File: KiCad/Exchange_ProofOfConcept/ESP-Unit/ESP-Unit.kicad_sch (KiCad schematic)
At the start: 52 parts, among them IC1 MT8870DE, J1 Jack-DC, J2 Conn_02x05_Top_Bottom, J3 Conn_01x07, U1 ESP32_NODEMCU, U2 LM317_TO-220, U3 LM358PE3, U4 BOB-12009, U5 BOB-12009, Y1 3.579546

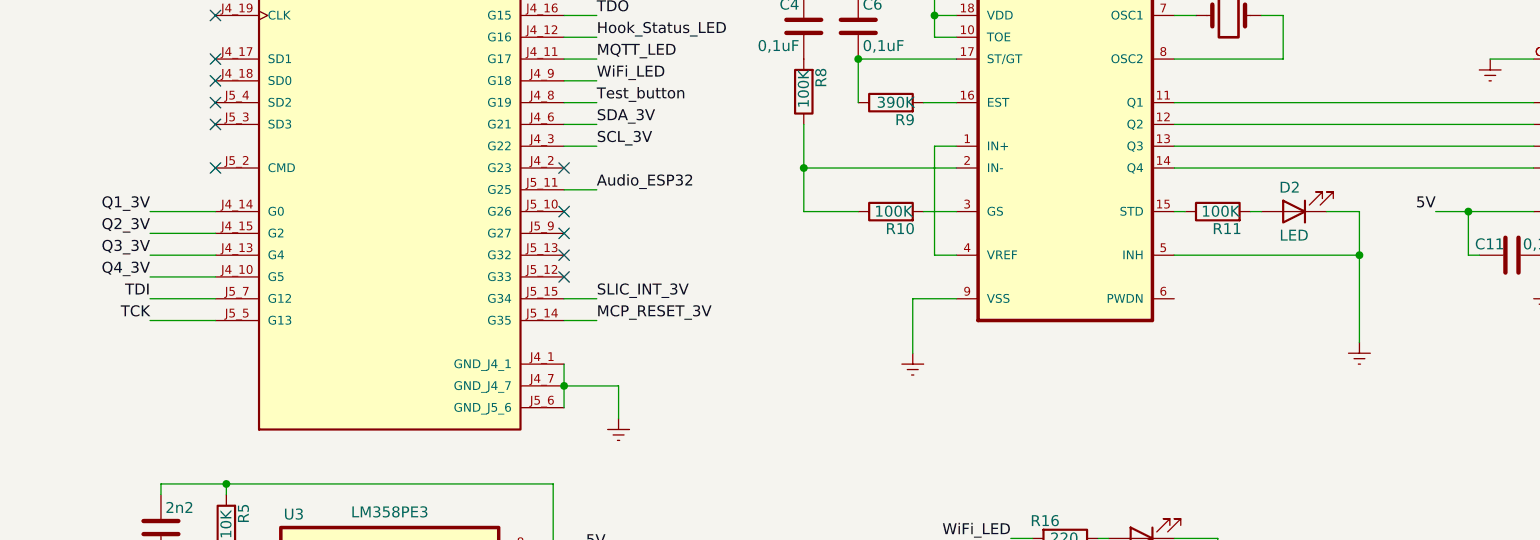
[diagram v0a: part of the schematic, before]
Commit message: modified:   KiCad/Exchange_ProofOfConcept/ESP-Unit/ESP-Unit.kicad_sch 	deleted:    KiCad/Exchange_ProofOfConcept/ESP-Unit/_autosave-ESP-Unit.kicad_sch 	modified:   include/config.h 	new file:   include/toneHandler.h 	modified:   lib/MT8816/MT8816.cpp 	modified:   src/config.cpp 	modified:   src/hookChange.cpp 	modified:   src/lineAction.cpp 	modified:   src/main.cpp 	new file:   src/toneHandler.cpp
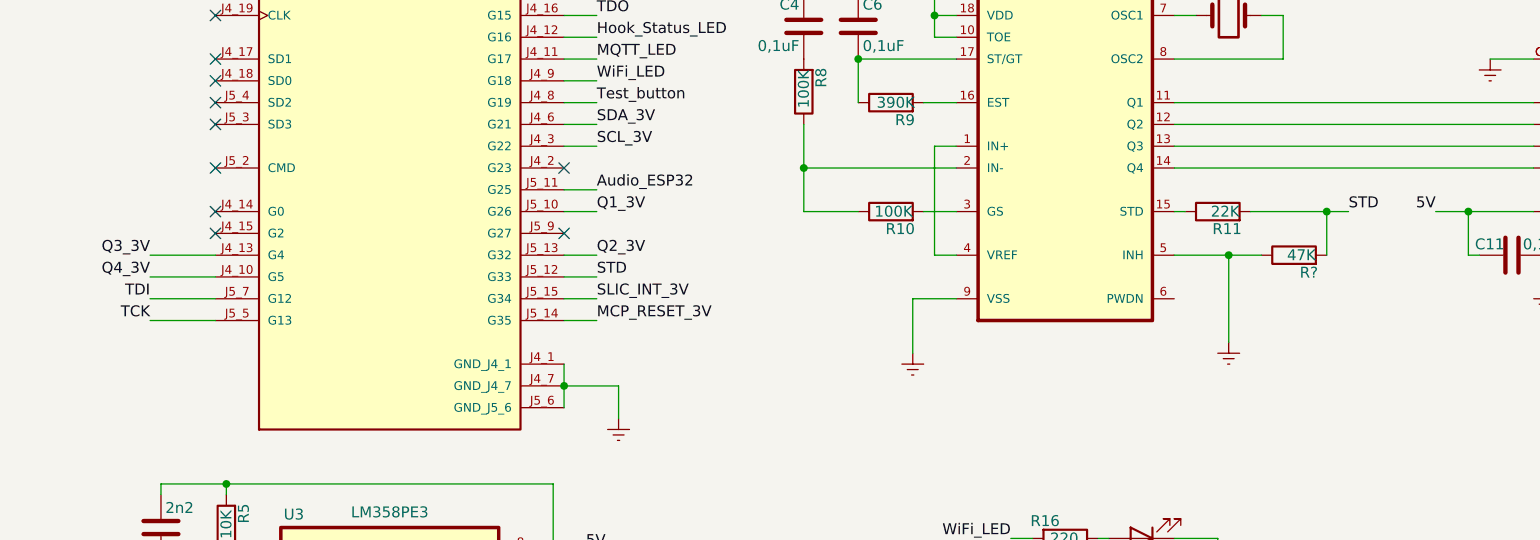
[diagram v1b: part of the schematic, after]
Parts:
- removed D2: LED, LED_THT:LED_D3.0mm, symbol Device:LED
- added R?: 47K, Resistor_THT:R_Axial_DIN0207_L6.3mm_D2.5mm_P2.54mm_Vertical, symbol Device:R
- R11: value 100K -> 22K
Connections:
- net Earth: now also R?.1
- net Q1_3V: now also U1.J5_10 (G26); no longer U1.J4_14 (G0)
- net Q2_3V: now also U1.J5_13 (G32); no longer U1.J4_15 (G2)
- net STD: now reaches R11.2
- net STD: now also U1.J5_12 (G33), R?.2
- no-connect marks 17 -> 16
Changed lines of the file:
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@@
 	)
 	(junction
+		(at 156.21 128.27)
+		(diameter 0)
+		(color 0 0 0 0)
+	)
+	(junction
 		(at 39.37 170.18)
 		(diameter 0)
@@
 	)
 	(junction
-		(at 171.45 128.27)
+		(at 167.64 123.19)
 		(diameter 0)
 		(color 0 0 0 0)
@@
 	)
 	(no_connect
+		(at 38.1 125.73)
+	)
+	(no_connect
 		(at 38.1 107.95)
 	)
@@
 	)
 	(no_connect
-		(at 78.74 128.27)
-	)
-	(no_connect
 		(at 38.1 92.71)
 	)
@@
 	)
 	(no_connect
-		(at 78.74 130.81)
-	)
-	(no_connect
 		(at 269.24 151.13)
 	)
@@
 	)
 	(no_connect
+		(at 38.1 123.19)
+	)
+	(no_connect
 		(at 38.1 118.11)
 	)
@@
 		(at 78.74 92.71)
 	)
-	(no_connect
-		(at 78.74 123.19)
-	)
 	(wire
 		(pts
@@
 	(wire
 		(pts
-			(xy 160.02 123.19) (xy 158.75 123.19)
+			(xy 158.75 123.19) (xy 167.64 123.19)
 		)
 		(stroke
@@
 	(wire
 		(pts
+			(xy 167.64 128.27) (xy 167.64 123.19)
+		)
+		(stroke
+			(width 0)
+			(type default)
+		)
+	)
+	(wire
+		(pts
 			(xy 107.95 46.99) (xy 107.95 58.42)
 		)
@@
 	(wire
 		(pts
-			(xy 149.86 128.27) (xy 171.45 128.27)
+			(xy 149.86 128.27) (xy 156.21 128.27)
 		)
 		(stroke
@@
 	(wire
 		(pts
-			(xy 30.48 123.19) (xy 38.1 123.19)
-		)
-		(stroke
-			(width 0)
-			(type default)
-		)
-	)
-	(wire
-		(pts
 			(xy 39.37 175.26) (xy 39.37 177.8)
 		)
@@
 	(wire
 		(pts
-			(xy 30.48 130.81) (xy 38.1 130.81)
+			(xy 167.64 123.19) (xy 170.18 123.19)
 		)
 		(stroke
@@
 	(wire
 		(pts
-			(xy 167.64 123.19) (xy 171.45 123.19)
+			(xy 30.48 130.81) (xy 38.1 130.81)
 		)
 		(stroke
@@
 	(wire
 		(pts
+			(xy 78.74 128.27) (xy 82.55 128.27)
+		)
+		(stroke
+			(width 0)
+			(type default)
+		)
+	)
+	(wire
+		(pts
 			(xy 248.92 73.66) (xy 248.92 83.82)
 		)
@@
 	(wire
 		(pts
+			(xy 78.74 123.19) (xy 82.55 123.19)
+		)
+		(stroke
+			(width 0)
+			(type default)
+		)
+	)
+	(wire
+		(pts
 			(xy 130.81 176.53) (xy 133.35 176.53)
 		)
@@
 	(wire
 		(pts
-			(xy 171.45 128.27) (xy 171.45 138.43)
+			(xy 156.21 128.27) (xy 156.21 138.43)
 		)
 		(stroke
@@
 	(wire
 		(pts
-			(xy 171.45 123.19) (xy 171.45 128.27)
+			(xy 31.75 165.1) (xy 39.37 165.1)
 		)
 		(stroke
@@
 	(wire
 		(pts
-			(xy 31.75 165.1) (xy 39.37 165.1)
+			(xy 78.74 130.81) (xy 82.55 130.81)
 		)
 		(stroke
@@
 	(wire
 		(pts
+			(xy 156.21 128.27) (xy 160.02 128.27)
+		)
+		(stroke
+			(width 0)
+			(type default)
+		)
+	)
+	(wire
+		(pts
 			(xy 120.65 110.49) (xy 124.46 110.49)
 		)
@@
 	(wire
 		(pts
-			(xy 30.48 125.73) (xy 38.1 125.73)
-		)
-		(stroke
-			(width 0)
-			(type default)
-		)
-	)
-	(wire
-		(pts
 			(xy 74.93 50.8) (xy 83.82 50.8)
 		)
@@
 		)
 	)
+	(label "STD"
+		(at 82.55 130.81 0)
+		(effects
+			(font
+				(size 1.27 1.27)
+			)
+			(justify left bottom)
+		)
+	)
 	(label "3V3"
 		(at 92.71 85.09 0)
@@
 		)
 	)
+	(label "STD"
+		(at 170.18 123.19 0)
+		(effects
+			(font
+				(size 1.27 1.27)
+			)
+			(justify left bottom)
+		)
+	)
 	(label "5V"
 		(at 118.11 86.36 180)
@@
 		)
 	)
-	(label "Q2_3V"
-		(at 30.48 125.73 180)
-		(effects
-			(font
-				(size 1.27 1.27)
-			)
-			(justify right bottom)
-		)
-	)
 	(label "Audio_SLIC-Amp"
 		(at 81.28 167.64 0)
@@
 		)
 	)
+	(label "Q1_3V"
+		(at 82.55 123.19 0)
+		(effects
+			(font
+				(size 1.27 1.27)
+			)
+			(justify left bottom)
+		)
+	)
 	(label "3V3"
 		(at 180.34 55.88 0)
@@
 		)
 	)
+	(label "Q2_3V"
+		(at 82.55 128.27 0)
+		(effects
+			(font
+				(size 1.27 1.27)
+			)
+			(justify left bottom)
+		)
+	)
 	(label "Audio_SLIC"
 		(at 248.92 71.12 0)
@@
 		)
 	)
-	(label "Q1_3V"
-		(at 30.48 123.19 180)
-		(effects
-			(font
-				(size 1.27 1.27)
-			)
-			(justify right bottom)
-		)
-	)
 	(label "Vref"
 		(at 134.62 31.75 0)
@@
 	)
 	(symbol
+		(lib_id "Device:R")
+		(at 163.83 128.27 90)
+		(unit 1)
+		(exclude_from_sim no)
+		(in_bom yes)
+		(on_board yes)
+		(dnp no)
+		(property "Reference" "R?"
+			(at 166.624 130.302 90)
+			(effects
+				(font
+					(size 1.27 1.27)
+				)
+				(justify left)
+			)
+		)
+		(property "Value" "47K"
+			(at 166.37 128.27 90)
+			(effects
+				(font
+					(size 1.27 1.27)
+				)
+				(justify left)
+			)
+		)
+		(property "Footprint" "Resistor_THT:R_Axial_DIN0207_L6.3mm_D2.5mm_P2.54mm_Vertical"
+			(at 163.83 130.048 90)
+			(effects
+				(font
+					(size 1.27 1.27)
+				)
+				(hide yes)
+			)
+		)
+		(property "Datasheet" "~"
+			(at 163.83 128.27 0)
+			(effects
+				(font
+					(size 1.27 1.27)
+				)
+				(hide yes)
+			)
+		)
+		(property "Description" "Resistor"
+			(at 163.83 128.27 0)
+			(effects
+				(font
+					(size 1.27 1.27)
+				)
+				(hide yes)
+			)
+		)
+		(pin "2"
+		)
+		(pin "1"
+		)
+		(instances
+			(project "ESP-Unit"
+				(path "/2411d7b8-ed2d-41a6-b5ea-3554d7cee414"
+					(reference "R?")
+					(unit 1)
+				)
+			)
+		)
+	)
+	(symbol
 		(lib_id "Device:C_Polarized_US")
 		(at 30.48 85.09 0)
@@
 	(symbol
 		(lib_id "power:Earth")
-		(at 171.45 138.43 0)
+		(at 156.21 138.43 0)
 		(mirror y)
 		(unit 1)
@@
 		(fields_autoplaced yes)
 		(property "Reference" "#PWR08"
-			(at 171.45 144.78 0)
+			(at 156.21 144.78 0)
 			(effects
 				(font
@@
 		)
 		(property "Value" "Earth"
-			(at 171.45 143.51 0)
+			(at 156.21 143.51 0)
 			(effects
 				(font
@@
 		)
 		(property "Footprint" ""
-			(at 171.45 138.43 0)
+			(at 156.21 138.43 0)
 			(effects
 				(font
@@
 		)
 		(property "Datasheet" "~"
-			(at 171.45 138.43 0)
+			(at 156.21 138.43 0)
 			(effects
 				(font
@@
 		)
 		(property "Description" "Power symbol creates a global label with name \"Earth\""
-			(at 171.45 138.43 0)
+			(at 156.21 138.43 0)
 			(effects
 				(font
@@
 	)
 	(symbol
-		(lib_id "Device:LED")
-		(at 163.83 123.19 180)
-		(unit 1)
-		(exclude_from_sim no)
-		(in_bom yes)
-		(on_board yes)
-		(dnp no)
-		(property "Reference" "D2"
-			(at 163.322 120.396 0)
-			(effects
-				(font
-					(size 1.27 1.27)
-				)
-			)
-		)
-		(property "Value" "LED"
-			(at 163.83 125.984 0)
-			(effects
-				(font
-					(size 1.27 1.27)
-				)
-			)
-		)
-		(property "Footprint" "LED_THT:LED_D3.0mm"
-			(at 163.83 123.19 0)
-			(effects
-				(font
-					(size 1.27 1.27)
-				)
-				(hide yes)
-			)
-		)
-		(property "Datasheet" "~"
-			(at 163.83 123.19 0)
-			(effects
-				(font
-					(size 1.27 1.27)
-				)
-				(hide yes)
-			)
-		)
-		(property "Description" "Light emitting diode"
-			(at 163.83 123.19 0)
-			(effects
-				(font
-					(size 1.27 1.27)
-				)
-				(hide yes)
-			)
-		)
-		(pin "1"
-		)
-		(pin "2"
-		)
-		(instances
-			(project "ESP-Unit"
-				(path "/2411d7b8-ed2d-41a6-b5ea-3554d7cee414"
-					(reference "D2")
-					(unit 1)
-				)
-			)
-		)
-	)
-	(symbol
 		(lib_id "Device:R")
 		(at 154.94 123.19 90)
@@
 			)
 		)
-		(property "Value" "100K"
+		(property "Value" "22K"
 			(at 157.48 123.19 90)
 			(effects
